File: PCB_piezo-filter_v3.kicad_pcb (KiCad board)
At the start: 2 copper layers, 115.5 x 39.5 mm, 48 parts, among them J1 Conn_01x02_Pin, J2 Conn_01x03_Pin, J3 Conn_01x01_Pin, J4 Conn_01x01_Pin, J5 Conn_01x01_Pin, J6 Conn_01x01_Pin, U1 TL062, U2 TLC2262CP, U3 TLC2262CP

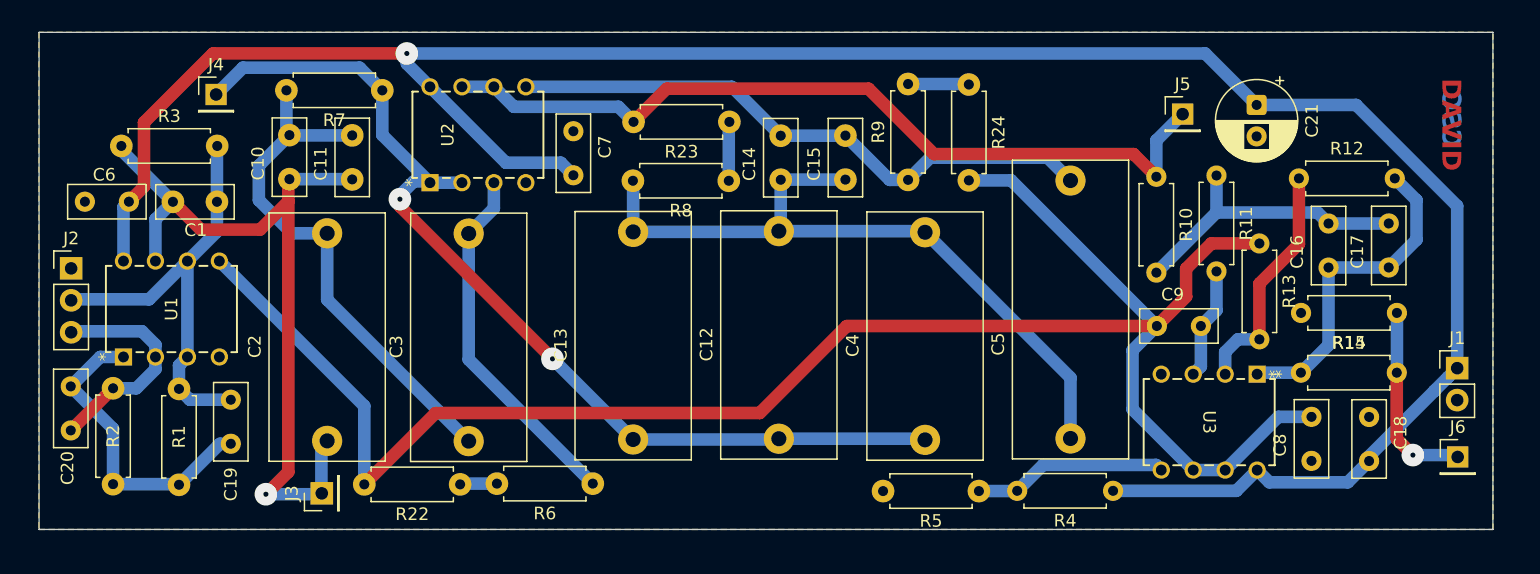
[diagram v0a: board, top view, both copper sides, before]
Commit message: update clearance to 1.6
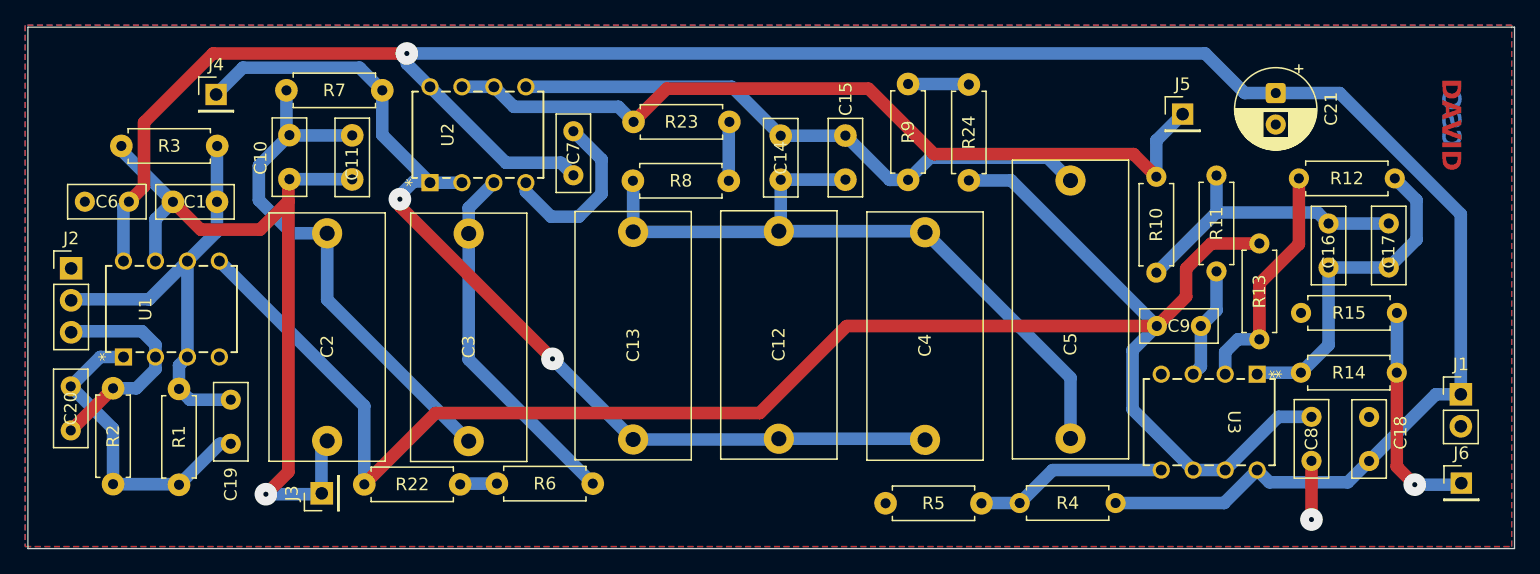
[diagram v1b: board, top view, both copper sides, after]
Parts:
- moved J1 2.10 mm to (223.8, 119.1)
- moved J6 2.10 mm to (223.9, 126.2)
- moved C21 1.79 mm to (209.1, 95.2)
- moved R4 0.99 mm to (196.4, 127.8)
- moved R5 0.99 mm to (185.7, 127.8)
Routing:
- net VEE: track 0.00 -> 18.9 mm, vias 0 -> 1
- net Net-(J6-Pin_1): track 15.5 -> 18.0 mm
- net VCC: track 186.4 -> 187.8 mm
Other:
- board size 115.5 x 39.5 mm -> 118.2 x 41.4 mm
